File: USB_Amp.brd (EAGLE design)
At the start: 80 x 72 mm, 140 parts, among them CON1 USB-C, CON2 PROG, CON3 DC IN, CON4 VOLUEME, CON5 SWD, IC1 3.3V, IC2 PIC32MZEF, IC3 SSM3582, IC4 +5V, IC5 1.8V, IC6 TL431, IC7 STM32G031F, IC8 +5V, IC9 3.3V, Q1 NPN, Q2 NPN, X1 24.576MHz, X2 22.5792MHz, X3 12MHz

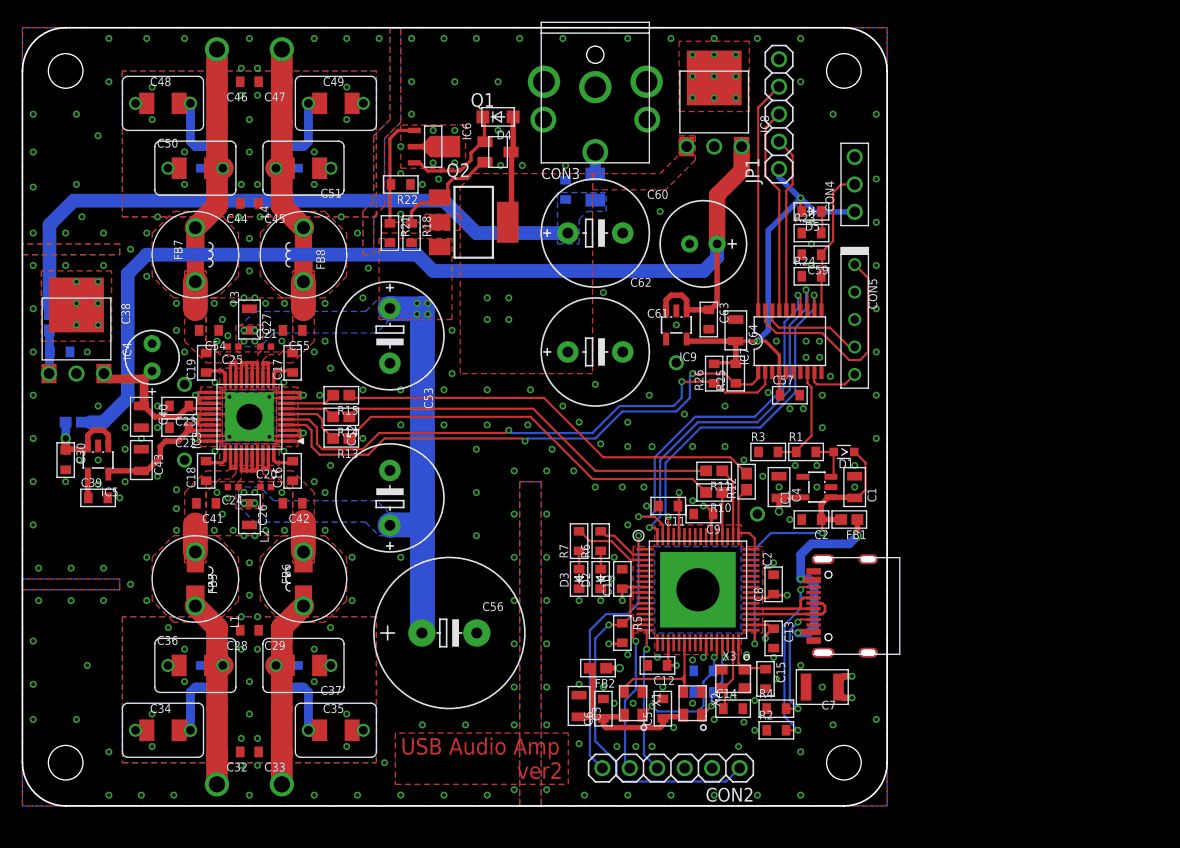
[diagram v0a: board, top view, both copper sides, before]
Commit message: 取り合えず
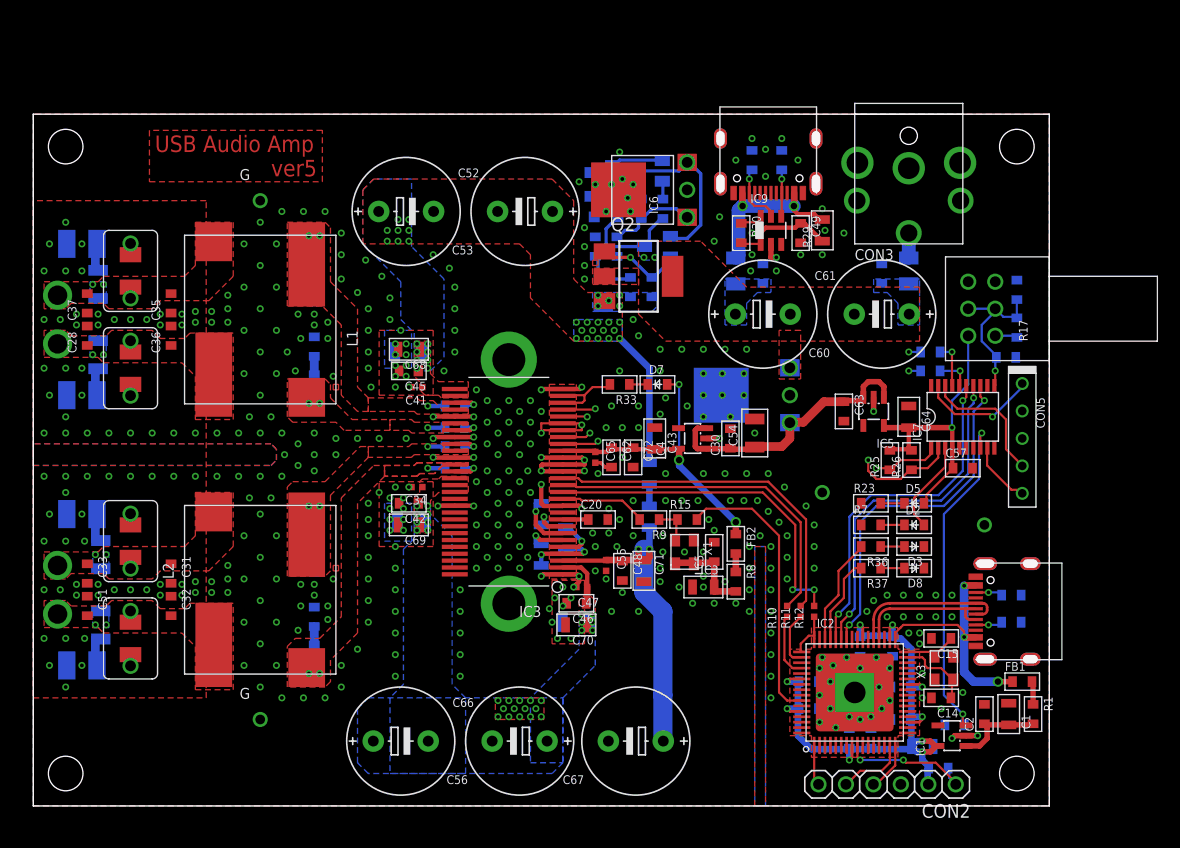
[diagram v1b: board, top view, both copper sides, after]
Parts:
- removed CON4: VOLUEME, my_connector:VOL_CON
- removed FB4: FB, my_rcl:1608-J
- removed FB5, FB6, FB7, FB8: FB, my_rcl:2012-FB
- removed JP1: IO, my_connector:1X05
- removed L3, L4: 15uH, my_rcl:L5-7,5
- removed X2: 22.5792MHz, my_rcl:KC3225
- added C65: 0.1u, my_rcl:1005
- added C66, C67: 470u, my_rcl:E5-10
- added C68, C69, C70, C71: 1u, my_rcl:2012
- added C72: 1u, my_rcl:1608C
- added C73, C77, C78, C79, C80: 100p, my_rcl:1608C
- added C74, C75, C76: 4.7u, my_rcl:3216
- added CON6: USB-C, my_connector:5077CR-16-SMC2-BK-TR
- added D6: 1mA, my_rcl:SOD123
- added D7: FAULT, my_rcl:D1608
- added D8: LED2, my_rcl:D1608
- added FB13: FB, my_rcl:3216-FB
- added HT1: HEATSINK-5, my_connector:V2199N1
- added Q3: PNP, my_ic:SC59
- added R27, R34, R35: 1k, my_rcl:1608
- added R28: DNP, my_rcl:1608
- added R29: 1k, my_rcl:2012
- added R30: 100k, my_rcl:1608
- added R31, R32: 5.1k, my_rcl:1608
- added R33, R36, R37: 3.3k, my_rcl:1608
- added R38, R39, R40, R41: 22, my_rcl:1608
- C14, C15: value 22p -> 10p
- C16, C17, C18, C19: value 0.22u -> 1u
- C20: value 10n -> 2.2u; device my_rcl:1005 -> my_rcl:1608C
- C21: value 10n -> 1u; device my_rcl:1005 -> my_rcl:2012
- C22, C23: value 0.1u -> 1u; device my_rcl:1608C -> my_rcl:2012
- C24, C25: device my_rcl:1005 -> my_rcl:3225-3
- C26, C40: value 10u -> 0.1u; device my_rcl:2012 -> my_rcl:3225-3
- C27: value 10u -> 0.47uF; device my_rcl:2012 -> my_rcl:C050W
- C29, C44: value 100p -> 0.47uF; device my_rcl:1608-2 -> my_rcl:C050W
- C31: value 0.1u -> 100p; device my_rcl:1608C -> my_rcl:1608-2
- C34: value 0.1u -> 10n; device my_rcl:C050W -> my_rcl:1005
- C35: value 0.1u -> 100p; device my_rcl:C050W -> my_rcl:1608-2
- C36, C37, C51: value 0.47uF -> 100p; device my_rcl:C050W -> my_rcl:1608-2
- C38: value 47u -> DNP; device my_rcl:E2.5-5 -> my_rcl:1608C
- C39: value 0.1u -> 10u; device my_rcl:1608C -> my_rcl:3216
- C41, C55: value DNP -> 10n; device my_rcl:1608-2 -> my_rcl:1005
- C42: value DNP -> 0.1u; device my_rcl:1608-2 -> my_rcl:1608C
- C45, C46: value 100p -> 0.1u; device my_rcl:1608-2 -> my_rcl:1608C
- C47: value 100p -> 10n; device my_rcl:1608-2 -> my_rcl:1005
- C48: device my_rcl:C050W -> my_rcl:1608C
- C49: value 0.1u -> 1u; device my_rcl:C050W -> my_rcl:1608C
- C50: value 0.47uF -> 0.1u; device my_rcl:C050W -> my_rcl:1608C
- C54: value DNP -> 10u; device my_rcl:1608-2 -> my_rcl:3216
- C56: value 1000u -> 470u; device my_rcl:E5-13 -> my_rcl:E5-10
- C59: value DNP -> 0.47uF; device my_rcl:1608C -> my_rcl:C050W
- C62: value 220u -> 1u; device my_rcl:E2,5-8 -> my_rcl:1608C
- C7: value 22u -> 1u; device my_rcl:3225 -> my_rcl:1608C
- CON3: value DC IN -> PWR IN
- D1: value SBD -> D; device my_rcl:SOD523 -> my_rcl:SOD323
- D4: value 5.6mA -> D; device my_rcl:SOD123 -> my_rcl:SOD323
- FB1, FB2: device my_rcl:1608-J -> my_rcl:1608-FB
- FB3: device my_rcl:1608-J -> my_rcl:2012-R
- IC3: value SSM3582 -> TAS6422; device my_ic:QFN40HT -> my_ic:HSSOP56-F
- IC4: value +5V -> 3.3V; device my_ic:TO220-SOP-DUAL -> my_ic:SOT23-5
- IC5: value 1.8V -> 3.3V
- IC6: device my_ic:SOT89 -> my_ic:TO220-SOP-DUAL
- IC7: value STM32G031F -> STM32G030F
- IC8: value +5V -> 7805
- IC9: value 3.3V -> CH221; device my_ic:SOT23-5 -> my_ic:SOT23-6
- L1, L2: value 15uH -> 10uH; device my_rcl:L5-7,5 -> my_rcl:UA8014
- R1: value 10k -> 5.1
- R10, R11, R12: device my_rcl:1608-J -> my_rcl:1005
- R13: value LRCLK -> 10; device my_rcl:1608-J -> my_rcl:3216-3
- R14: value DATA -> 10; device my_rcl:1608-J -> my_rcl:3216-3
- R15: value SCK -> 39; device my_rcl:1608-J -> my_rcl:1608
- R16: value 10 -> 100; device my_rcl:2012 -> my_rcl:1608
- R17: value 10 -> 50k; device my_rcl:2012 -> my_rcl:RK0972
- R19, R20: device my_rcl:2012 -> my_rcl:3216-3
- R23: value 10k -> 3.3k
- R3: value 10k -> 10; device my_rcl:1608 -> my_rcl:2012-R
- R6: value 1k -> 10k
- R7: value 1k -> 3.3k
- R8: value 10k -> 10
- R9: value 10k -> 39
- TP1, TP2: device my_connector:TESTPIN-BIG -> my_connector:TESTPIN-LARGE
- TP3: value R_P -> R_N; device my_connector:TESTPIN-BIG -> my_connector:TESTPIN-LARGE
- TP4: value R_N -> R_P; device my_connector:TESTPIN-BIG -> my_connector:TESTPIN-LARGE
- X3: device my_rcl:KC3225-2 -> my_rcl:KC3225-CRYSTAL
- moved R17 73.1 mm to (90.0, 46.0), flipped to the top
- moved IC5 71.9 mm to (78.8, 36.5)
- moved C59 68.3 mm to (10.0, 24.5), turned to 270 degrees
- moved C30 61.5 mm to (65.5, 34.0), turned to 90 degrees
- moved C48 60.6 mm to (55.5, 21.8), turned to 270 degrees
- moved R16 60.6 mm to (59.2, 55.2)
- moved C46 57.9 mm to (51.2, 18.8)
- moved IC4 57.3 mm to (62.0, 34.0), turned to 90 degrees
- moved C47 55.0 mm to (51.8, 20.2)
- moved TP4 54.3 mm to (3.25, 17.8)
- moved FB3 54.0 mm to (58.0, 26.8), turned to 270 degrees
- moved C50 53.4 mm to (68.5, 49.2), flipped to the bottom, turned to 90 degrees
- moved TP3 52.1 mm to (3.25, 22.2)
- moved C54 51.4 mm to (67.8, 34.5), turned to 90 degrees
- moved C39 50.5 mm to (53.8, 47.5), flipped to the bottom, turned to 90 degrees
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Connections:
- removed net +12V: C20.1, C21.1, C24.1, C25.1, C26.1, C27.1, C52.+, C53.+, C56.+, IC3.14, IC3.15, IC3.16, IC3.17, IC3.34, IC3.35, IC3.36, IC3.37, Q2.3, R18.2, R21.2
- removed net AMP_AVDD: C23.1, C38.+, C40.1, IC3.24, IC4.3, IC4.6
- removed net EN_44.1K: IC2.29, R9.2, X2.1
- removed net EN_48K: IC2.28, R8.2, X1.1
- removed net MCLK: IC2.22, X1.3, X2.3
- removed net STM_IO16: IC7.16, JP1.2
- removed net STM_IO17: IC7.17, JP1.3
- removed net STM_IO20: IC7.20, JP1.4
- new net AMP_FAULT: IC3.26, IC3.27, R33.2
- new net AMP_MUTE: IC3.25, R35.1
- new net AMP_STANBY: IC3.24, R34.1
- new net I2S_MCLK: IC3.12, R9.2
- new net LED2: IC2.45, R37.2
- new net N$25: C26.1, R13.1
- new net N$26: FB2.2, R8.1
- new net N$27: R15.1, R9.1, X1.3
- new net N$28: FB3.1, R3.2
- new net N$29: Q3.2, R16.1
- new net N$32: CON6.B5:CC2, IC9.5, R32.1
- new net N$33: C49.1, IC9.1, R29.1, R30.2
- new net N$34: IC9.6, R30.1
- new net N$35: D7.K, R33.1
- new net N$37: D1.1, D4.2
- new net N$38: D1.2, D6.1, Q3.1
- new net N$39: IC7.16, R35.2
- new net N$42: IC7.17, R34.2
- new net N$44: D8.A, R37.1
- new net N$45: C77.1, R38.1
- new net N$46: C78.2, R39.2
- new net N$47: C79.2, R40.2
- new net N$48: C80.1, R41.1
- new net N$6: C19.2, IC3.31
- new net PIC_MCLK: IC2.58, R15.2
- new net PVDD: C34.1, C39.1, C41.1, C42.1, C45.1, C46.1, C47.1, C52.+, C53.+, C56.+, C66.+, C68.1, C69.1, C70.1, C74.1, C75.1, C76.1, IC3.2, IC3.29, IC3.30, IC3.42, IC3.43, Q2.3, R18.2, R21.2, R3.1
- new net VBAT: C48.1, C55.1, C67.+, C71.1, FB3.2, IC3.3
- new net VINC_+: CON6.A4,B9:VBUS, CON6.B4,A9:VBUS, FB13.1, R29.2
- net +3V3: now also IC5.5, R17.1, R17.4, R28.2; no longer CON4.1, IC9.5, JP1.1
- net +3V3D: now also C6.1; no longer FB2.1
- net +5V: now also C30.1, C54.1, IC4.1, IC4.3, IC5.1, IC5.3; no longer C62.+, FB3.1, IC9.1, IC9.3
- net AMP_DVDD: now also C62.1, C65.1, C72.1, D7.A, FB2.1, IC3.19, IC4.5; no longer C22.1, IC3.28, IC5.5
- net AMP_OUTN_L: now also C19.1, R40.1; no longer C18.1, C41.2, FB5.2, IC3.33
- net AMP_OUTN_R: now also C17.1, IC3.38, L2.3, R38.2; no longer C19.2, C54.2, FB7.2, IC3.18, IC3.19, L3.2
- net AMP_OUTP_L: now also C18.2, IC3.34, L1.4, R41.2; no longer C16.1, C42.1, FB6.1, IC3.38, IC3.39, L2.2
- net AMP_OUTP_R: now also C16.2, IC3.40, L2.2, R39.1; no longer C17.2, C55.1, FB8.1, IC3.12, IC3.13, L4.1
- net EN_DDC: now also IC1.3, R6.1; no longer R1.1, R3.2
- net GND: now also C24.1, C25.1, C27.1, C27.3, C28.2, C29.1, C29.3, C34.2, C35.1, C36.2, C41.2, C44.3, C46.2, C48.2, C50.2, C54.2, C59.1, C59.3, C62.2, C65.2, C66.-, C67.-, C68.2, C69.2, C70.2, C71.2, C72.2, C73.2, C74.2, C75.2, C76.2, C77.2, C78.1, C79.1, C80.2, CON6.A1,B12:GND, CON6.B1,A12:GND, CON6.SHILED1, CON6.SHILED2, CON6.SHILED3, CON6.SHILED4, CON6.SHILED5, CON6.SHILED6, CON6.SHILED7, CON6.SHILED8, D6.2, D8.K, HT1.HT1, HT1.HT2, IC2.HT2, IC3.11, IC3.16, IC3.17, IC3.18, IC3.28, IC3.33, IC3.36, IC3.39, IC3.46, IC6.5, R17.3, R17.6, R31.2, R32.2, R6.2, R7.1; no longer C21.2, C22.2, C23.2, C24.2, C25.2, C27.2, C28.1, C29.2, C34.1, C34.3, C35.2, C35.4, C36.1, C36.3, C37.3, C38.-, C39.2, C41.1, C46.1, C48.1, C48.3, C49.4, C50.1, C50.3, C51.3, C54.1, C59.2, C62.-, CON4.3, D2.K, IC3.10, IC3.2, IC3.21, IC3.25, IC3.26, IC3.27, IC3.29, IC3.3, IC3.30, IC3.9, IC3.HT, IC3.HT1, IC3.HT2, IC3.HT3, IC3.HT4, IC4.5, JP1.5, R3.1, R8.1, R9.1, X2.2
- net I2C_SCL: now also IC3.20; no longer IC3.4
- net I2C_SDA: now also IC3.21; no longer IC3.5
- net I2S_DATA: now also IC3.15; no longer R14.1
- net I2S_LRCLK: now also IC3.14; no longer R13.1
- net I2S_SCK: now also IC3.13; no longer R15.1
- net LED0: now also D2.A, IC7.3; no longer IC2.2, R6.2
- net LED1: now also IC2.46, R36.2; no longer IC2.3, R7.2
- net N$10: now also C20.1, IC3.9; no longer IC3.6, R13.2
- net N$11: now also C21.2, IC3.8; no longer IC3.7, R14.2
- net N$12: now also C21.1, IC3.7; no longer C18.2, IC3.31
- net N$13: now also C22.1, C23.1, IC3.4; no longer C16.2, IC3.40
- net N$14: now also C18.1, IC3.35; no longer IC3.8, R15.2
- net N$15: now also C22.2, IC3.6; no longer C39.1, IC5.4
- net N$17: now also C17.2, IC3.37; no longer C17.1, IC3.11
- net N$18: now also C23.2, IC3.5; no longer C19.1, IC3.20
- net N$19: now also C16.1, IC3.41; no longer C30.1, FB3.2, IC5.1, IC5.3
- net N$20: now also C38.2, IC6.4, R27.1; no longer R21.1, R22.2
- net N$21: now also C24.2, R19.2; no longer C34.2, C34.4, R16.2
- net N$22: now also C40.1, R20.1; no longer C35.1, C35.3, R17.1
- net N$23: now also C38.1, IC6.6, Q3.3; no longer D4.2
- net N$24: now also C25.2, R14.2; no longer C31.1, FB4.2, IC4.1, IC4.4
- net N$3: now also FB1.2, R1.1; no longer CON1.A4,B9:VBUS, CON1.B4,A9:VBUS, FB1.1
- net N$30: now also C39.2, R21.1, R22.2, R27.2; no longer C48.2, C48.4, R19.2
- net N$31: now also CON6.A5:CC1, IC9.4, R31.1; no longer C49.1, C49.3, R20.1
- net N$4: now also C1.1, C2.1, IC1.1; no longer D1.A, IC1.3
- net N$72: now also C73.1, R17.2, R17.5, R28.1; no longer C59.1, CON4.2
- net N$8: now also D2.K, R7.2; no longer D2.A, R6.1
- net N$9: now also R36.1; no longer R7.1
- net PIC_COM1: now also IC2.44, IC7.15; no longer IC2.62, IC7.12
- net PIC_COM2: now also IC2.43, IC7.14; no longer IC2.64, IC7.13
- net PIC_COM3: now also IC2.42, IC7.13; no longer IC2.63, IC7.14
- net SP_OUTN_L: now also C27.2, C27.4, C35.2, C37.2, R19.1; no longer C28.2, C32.2, C36.2, C36.4, FB5.1, R16.1
- net SP_OUTN_R: now also C31.1, C33.1, C59.2, C59.4, L2.4, R13.2, TP3.1; no longer C44.2, C46.2, C50.2, C50.4, FB7.1, L3.1, R19.1, TP4.1
- net SP_OUTP_L: now also C28.1, C36.1, C44.2, C44.4, L1.3, R20.2; no longer C29.1, C33.1, C37.2, C37.4, FB6.2, L2.1, R17.2
- net SP_OUTP_R: now also C29.2, C29.4, C32.2, L2.1, R14.1, TP4.1; no longer C45.1, C47.1, C51.4, FB8.2, L4.2, R20.2, TP3.1
- net USB_VBUS: now also CON1.A4,B9:VBUS, CON1.B4,A9:VBUS, FB1.1; no longer C1.1, C2.1, D1.K, FB1.2, IC1.1
- net V+: now also C50.1, FB13.2, R16.2; no longer FB4.1
- net XVCC: now also R8.2, X1.1; no longer C6.1, FB2.2, X2.4
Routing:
- net +5V: track 97.1 -> 25.6 mm
- net V+: track 68.4 -> 10.0 mm, vias 0 -> 2
- net +12V: track 51.8 -> 0.00 mm, vias 12 -> 0
- net AMP_MUTE: track 0.00 -> 38.6 mm, vias 0 -> 2
- net AMP_STANBY: track 0.00 -> 38.6 mm, vias 0 -> 2
- net VBAT: track 0.00 -> 31.8 mm, vias 0 -> 2
- net PIC_MCLK: track 0.00 -> 26.0 mm
- net +3V3D: track 32.3 -> 58.3 mm, vias 12 -> 9
- net UART_TX: track 26.9 -> 3.77 mm, vias 1 -> 0
- net SP_OUTP_R: track 22.6 -> 0.00 mm, vias 0 -> 2
- net SP_OUTN_R: track 22.5 -> 0.00 mm, vias 0 -> 2
- net SP_OUTP_L: track 22.3 -> 0.00 mm, vias 0 -> 2
- net SP_OUTN_L: track 22.2 -> 0.00 mm, vias 0 -> 2
- net EN_DDC: track 9.84 -> 31.8 mm, vias 0 -> 2
- net STM_IO20: track 21.5 -> 0.00 mm
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- added copper zone on layer 16, net AMP_OUTN_L
- added copper zone on layer 16, net AMP_OUTN_R
- added copper zone on layer 16, net AMP_OUTP_L
- added copper zone on layer 16, net AMP_OUTP_R
- added copper zone on layer 1, net PVDD
- added copper zone on layer 16, net PVDD
- added copper zone on layer 1, net SP_OUTN_L
- added copper zone on layer 16, net SP_OUTN_L
- added copper zone on layer 1, net SP_OUTN_R
- added copper zone on layer 16, net SP_OUTN_R
- added copper zone on layer 1, net SP_OUTP_L
- added copper zone on layer 16, net SP_OUTP_L
- added copper zone on layer 1, net SP_OUTP_R
- added copper zone on layer 16, net SP_OUTP_R
- removed copper zone on layer 1, net +12V
- removed copper zone on layer 16, net +12V
- removed copper zone on layer 15, net +3V3D
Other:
- board size 80 x 72 mm -> 94 x 64 mm
- board text added: "ver5"
- board text removed: "ver2"
